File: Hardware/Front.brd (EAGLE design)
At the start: 100 x 17 mm, 60 parts, among them IC3 MAX6951

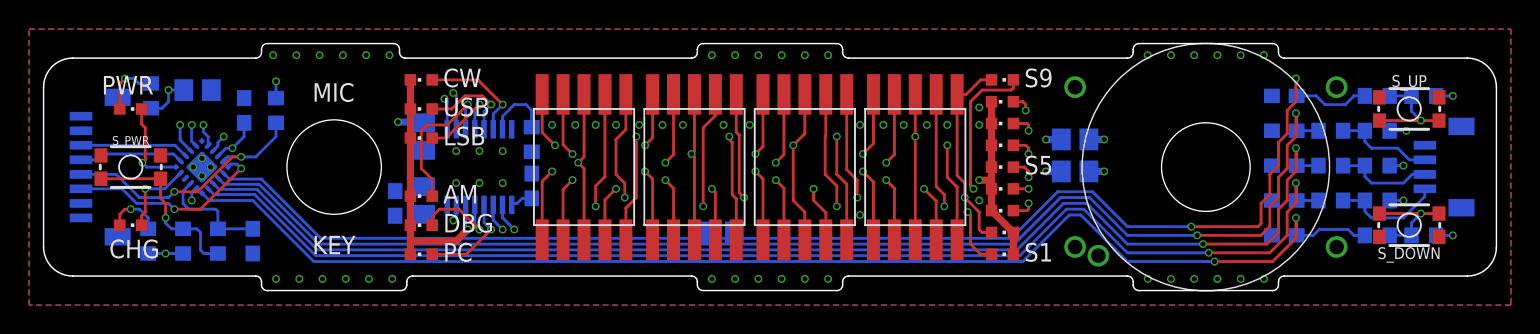
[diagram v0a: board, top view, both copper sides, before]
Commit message: Finish version 0.1 of front
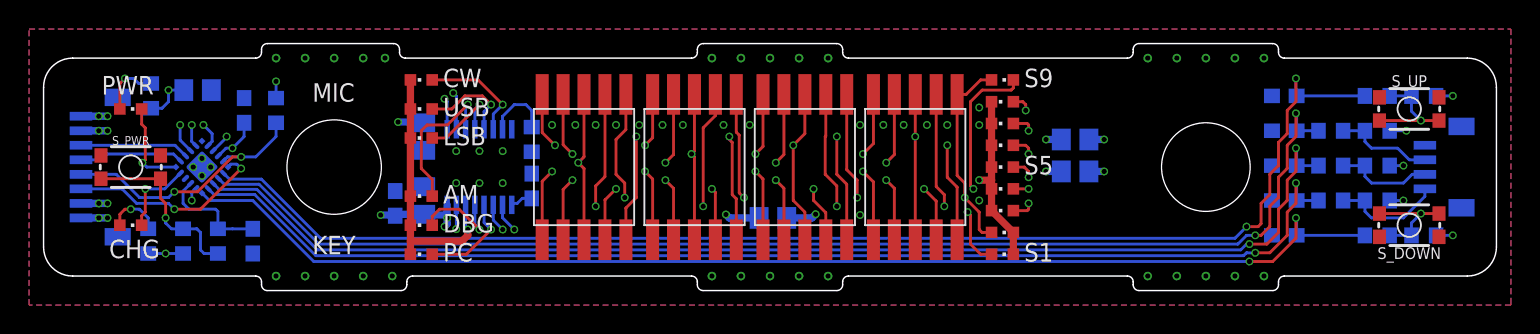
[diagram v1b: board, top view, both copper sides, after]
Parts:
- moved C15 3.74 mm to (50.2, 5.00)
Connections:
- net GND: now also U$1.GND@10, U$1.GND@11, U$1.GND@12, U$1.GND@13, U$1.GND@14, U$1.GND@15, U$1.GND@16, U$1.GND@17, U$1.GND@18, U$1.GND@19, U$1.GND@20, U$1.GND@21, U$1.GND@22, U$1.GND@23, U$1.GND@24, U$1.GND@25, U$1.GND@26, U$1.GND@27, U$1.GND@28, U$1.GND@29, U$1.GND@3, U$1.GND@30, U$1.GND@4, U$1.GND@5, U$1.GND@6, U$1.GND@7, U$1.GND@8, U$1.GND@9; no longer U$1.GND, U$1.GND2
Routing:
- net +3V3: track 19.6 -> 31.8 mm, vias 12 -> 20
- net GND: track 4.49 -> 10.7 mm, vias 64 -> 37
- net BTN_DWN: track 88.2 -> 85.2 mm
- net BTN_UP: track 93.1 -> 90.6 mm
- net ENC_A: track 85.8 -> 83.3 mm
- net ENC_B: track 87.0 -> 84.7 mm
- net ENC_C: track 88.2 -> 86.0 mm
- net SPI_!CS: track 30.2 -> 31.2 mm
